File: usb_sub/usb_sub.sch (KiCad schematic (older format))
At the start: 23 parts, among them P3 CONN_2, U1 AURORA_CARD, U2 MICRO-B_USB, U3 FT232RQ, U4 AP7333, U5 LD1117

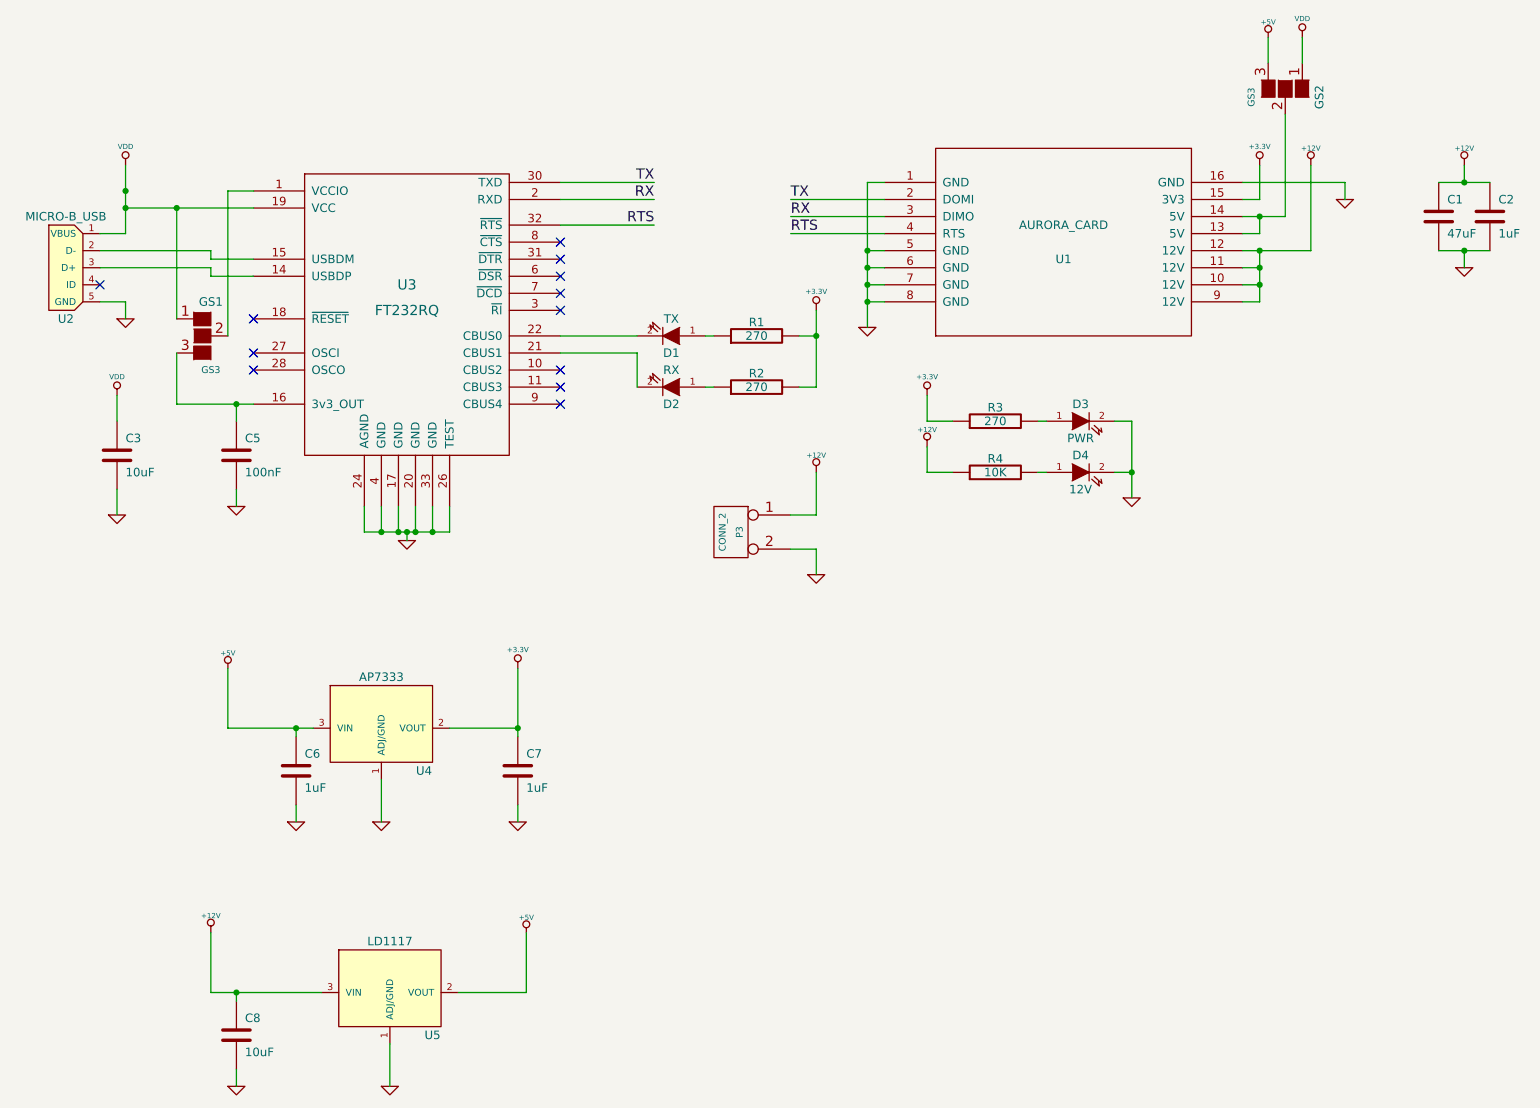
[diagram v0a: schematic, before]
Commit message: Debugging router
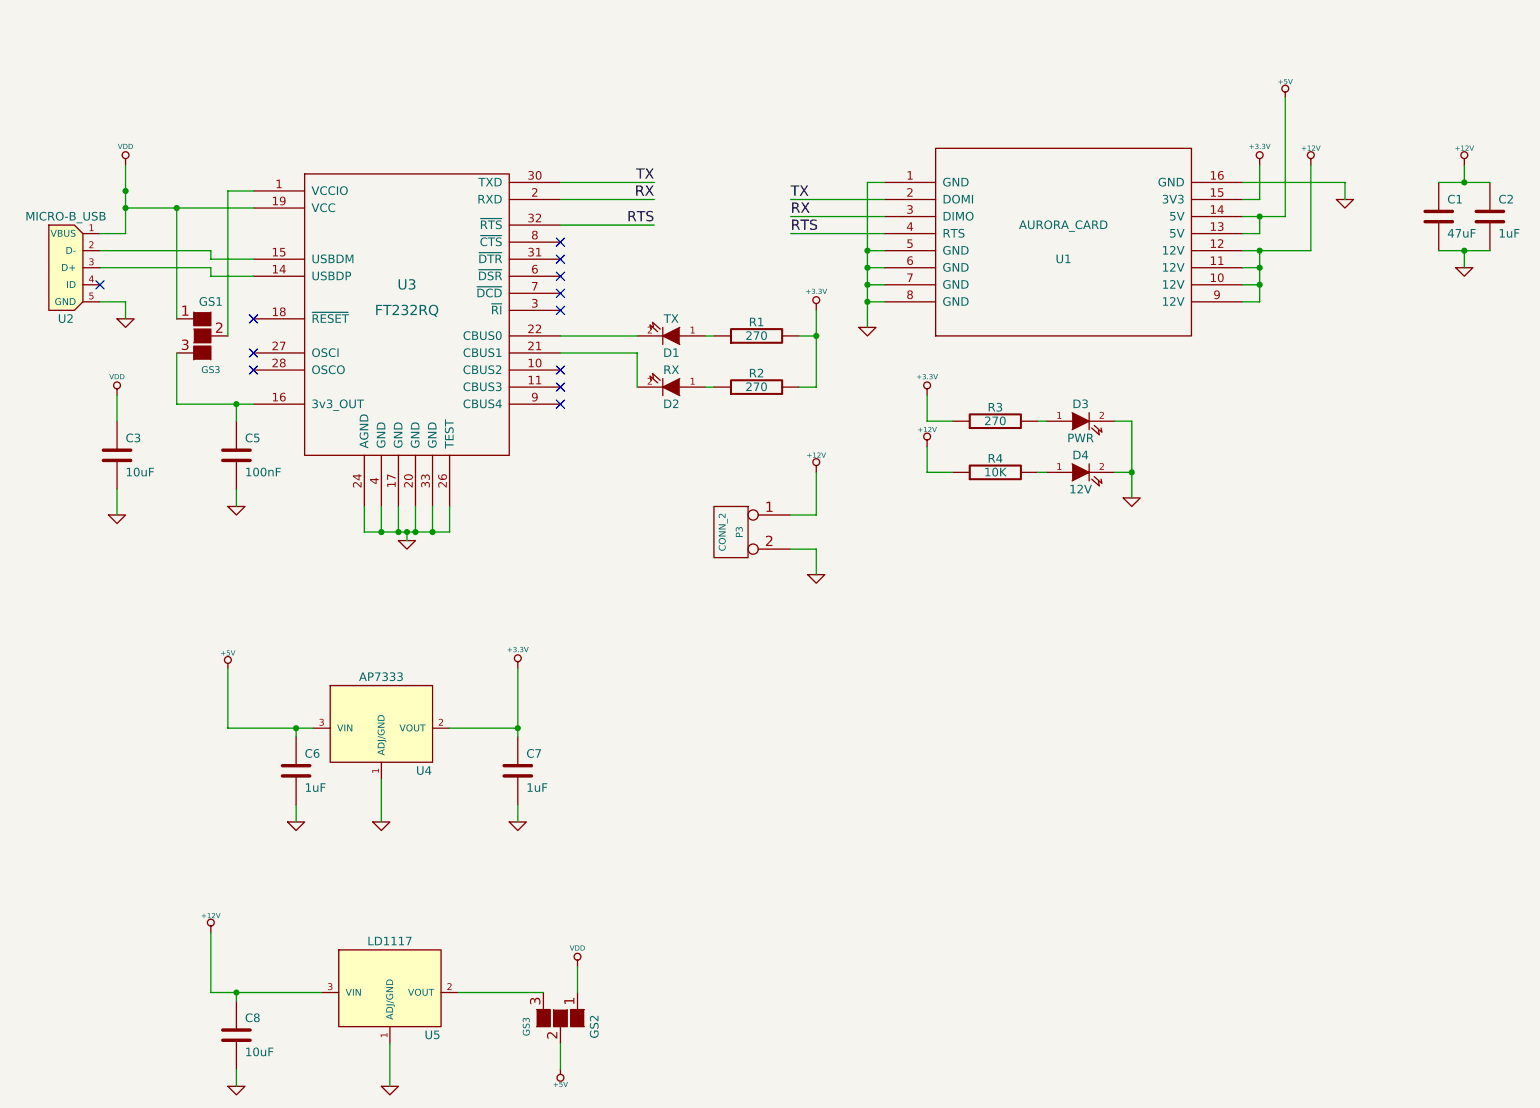
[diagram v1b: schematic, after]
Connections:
- net +5V: now also GS2.2 (G2), U1.13 (5V), U1.14 (5V); no longer GS2.3 (G3), U5.2 (VOUT)
- new net: GS2.3 (G3), U5.2 (VOUT)
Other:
- moved on the sheet: GS2
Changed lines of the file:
@@
 	5500 2950 5400 2950
-Wire Wire Line
-	3800 6450 3800 6800
 Wire Wire Line
 	1400 3850 1400 4000
@@
 	1950 6800 2600 6800
 Wire Wire Line
-	3800 6800 3400 6800
+	3400 6800 3900 6800
 Wire Wire Line
 	2450 5800 2450 5700
@@
 L +5V #PWR06
 U 1 1 52C95643
-P 8150 1200
-F 0 "#PWR06" H 8150 1290 20  0001 C CNN
-F 1 "+5V" H 8150 1290 30  0000 C CNN
-F 2 "" H 8150 1200 60  0001 C CNN
-F 3 "" H 8150 1200 60  0001 C CNN
-	1    8150 1200
-	1    0    0    -1
+P 4000 7250
+F 0 "#PWR06" H 4000 7340 20  0001 C CNN
+F 1 "+5V" H 4000 7340 30  0000 C CNN
+F 2 "" H 4000 7250 60  0001 C CNN
+F 3 "" H 4000 7250 60  0001 C CNN
+	1    4000 7250
+	-1   0    0    1
 $EndComp
 $Comp
@@
 F 3 "" H 3000 7350 60  0001 C CNN
 	1    3000 7350
-	1    0    0    -1
-$EndComp
-$Comp
-L +5V #PWR015
-U 1 1 52C933EC
-P 3800 6450
-F 0 "#PWR015" H 3800 6540 20  0001 C CNN
-F 1 "+5V" H 3800 6540 30  0000 C CNN
-F 2 "" H 3800 6450 60  0001 C CNN
-F 3 "" H 3800 6450 60  0001 C CNN
-	1    3800 6450
 	1    0    0    -1
 $EndComp
@@
 L GS3 GS2
 U 1 1 53B4301E
-P 8250 1500
-F 0 "GS2" H 8300 1700 50  0000 C CNN
-F 1 "GS3" H 8300 1301 40  0000 C CNN
-F 2 "" H 8250 1500 60  0001 C CNN
-F 3 "" H 8250 1500 60  0001 C CNN
-	1    8250 1500
+P 4000 6950
+F 0 "GS2" H 4050 7150 50  0000 C CNN
+F 1 "GS3" H 4050 6751 40  0000 C CNN
+F 2 "" H 4000 6950 60  0001 C CNN
+F 3 "" H 4000 6950 60  0001 C CNN
+	1    4000 6950
 	0    1    1    0
 $EndComp
-Wire Wire Line
-	8150 1200 8150 1350
-Wire Wire Line
-	8250 2250 8250 1650
 $Comp
 L VDD #PWR028
 U 1 1 53B4313A
-P 8350 1200
-F 0 "#PWR028" H 8350 1300 30  0001 C CNN
-F 1 "VDD" H 8350 1310 30  0000 C CNN
-F 2 "" H 8350 1200 60  0000 C CNN
-F 3 "" H 8350 1200 60  0000 C CNN
-	1    8350 1200
-	1    0    0    -1
-$EndComp
-Wire Wire Line
-	8350 1200 8350 1350
+P 4100 6650
+F 0 "#PWR028" H 4100 6750 30  0001 C CNN
+F 1 "VDD" H 4100 6760 30  0000 C CNN
+F 2 "" H 4100 6650 60  0000 C CNN
+F 3 "" H 4100 6650 60  0000 C CNN
+	1    4100 6650
+	1    0    0    -1
+$EndComp
+Wire Wire Line
+	4100 6650 4100 6800
 $Comp
 L FT232RQ U3
@@
 $EndComp
 Wire Wire Line
-	3100 4150 3100 4100
+	3100 4100 3100 4150
 Wire Wire Line
 	2850 4100 3350 4100
@@
 NoConn ~ 4000 3350
 NoConn ~ 1300 2650
+Wire Wire Line
+	4000 7250 4000 7100
+$Comp
+L +5V #PWR?
+U 1 1 53D4111B
+P 8250 1550
+F 0 "#PWR?" H 8250 1640 20  0001 C CNN
+F 1 "+5V" H 8250 1640 30  0000 C CNN
+F 2 "" H 8250 1550 60  0001 C CNN
+F 3 "" H 8250 1550 60  0001 C CNN
+	1    8250 1550
+	1    0    0    -1
+$EndComp
+Wire Wire Line
+	8250 2250 8250 1550
 $EndSCHEMATC
